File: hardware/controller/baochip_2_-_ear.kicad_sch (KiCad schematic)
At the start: 16 parts, among them U3 EA8212HT6R, U4 EA8212HT6R

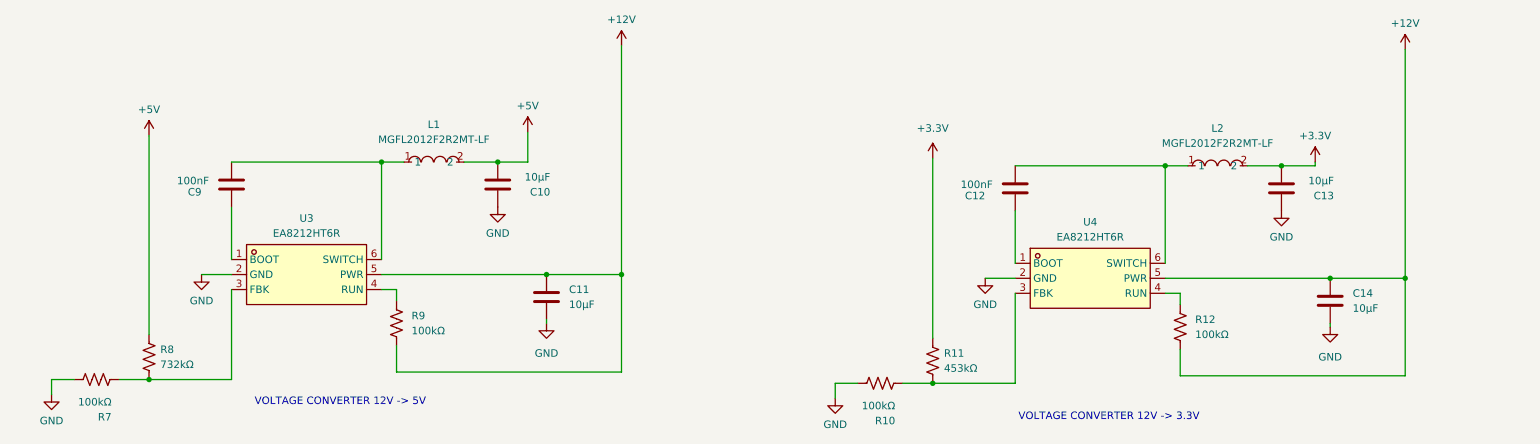
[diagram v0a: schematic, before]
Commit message: more controller board work, consolidation/revision of design
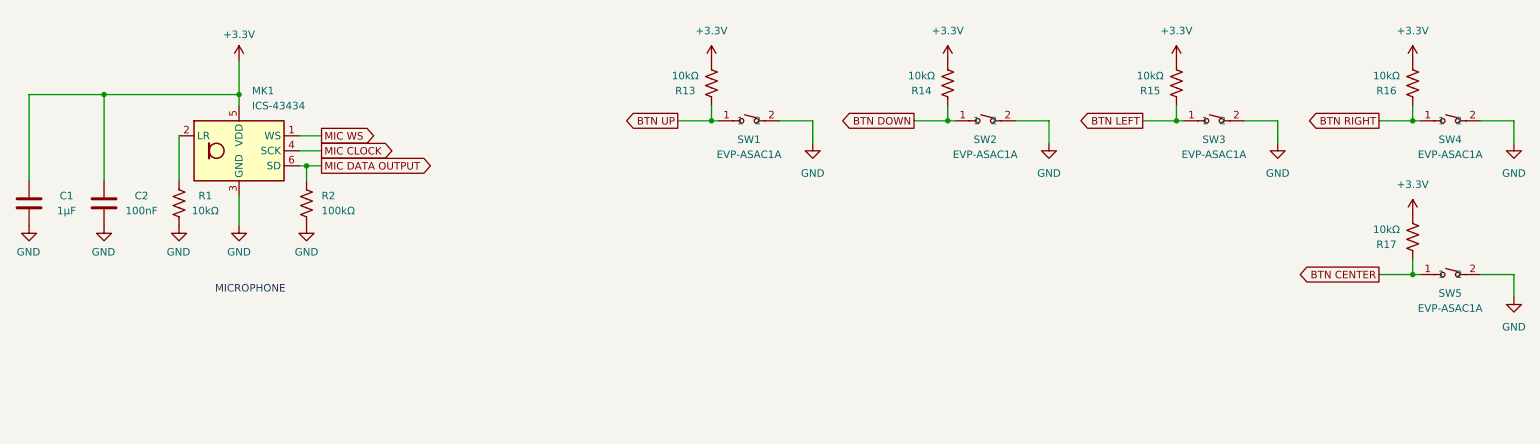
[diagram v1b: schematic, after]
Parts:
- removed C10, C11, C13, C14: 10µF, Capacitor_SMD:C_0603_1608Metric, symbol Device:C
- removed C12, C9: 100nF, Capacitor_SMD:C_0402_1005Metric, symbol Device:C
- removed L1, L2: MGFL2012F2R2MT-LF, footprints:L0805, symbol easyeda2kicad:MGFL2012F2R2MT-LF
- removed R10, R12, R7, R9: 100kΩ, Resistor_SMD:R_0402_1005Metric, symbol Device:R_US
- removed R11: 453kΩ, Resistor_SMD:R_0402_1005Metric, symbol Device:R_US
- removed R8: 732kΩ, Resistor_SMD:R_0402_1005Metric, symbol Device:R_US
- removed U3, U4: EA8212HT6R, footprints:SOT-23-6_L2.9-W1.6-P0.95-LS2.8-BR, symbol new:EA8212HT6R
- added C1: 1µF, Capacitor_SMD:C_0603_1608Metric, symbol Device:C
- added C2: 100nF, Capacitor_SMD:C_0402_1005Metric, symbol Device:C
- added MK1: ICS-43434, Sensor_Audio:InvenSense_ICS-43434-6_3.5x2.65mm, symbol Sensor_Audio:ICS-43434
- added R1, R13, R14, R15, R16, R17: 10kΩ, Resistor_SMD:R_0603_1608Metric, symbol Device:R_US
- added R2: 100kΩ, Resistor_SMD:R_0603_1608Metric, symbol Device:R_US
- added SW1, SW2, SW3, SW4, SW5: EVP-ASAC1A, easyeda2kicad:SW-SMD_PANASONIC_EVPASXXX, symbol easyeda2kicad:EVP-ASAC1A
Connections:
- net +3.3V: now also C1.1, C2.1, MK1.5 (VDD), R13.1, R14.1, R15.1, R16.1, R17.1
- net GND: now also C1.2, C2.2, MK1.3 (GND), R1.1, R2.1, SW1.2, SW2.2, SW3.2, SW4.2, SW5.2
- new net: MK1.2 (LR), R1.2
- new net BTN CENTER: R17.2, SW5.1
- new net BTN DOWN: R14.2, SW2.1
- new net BTN LEFT: R15.2, SW3.1
- new net BTN RIGHT: R16.2, SW4.1
- new net BTN UP: R13.2, SW1.1
- new net MIC CLOCK: MK1.4 (SCK)
- new net MIC DATA OUTPUT: MK1.6 (SD), R2.2
- new net MIC WS: MK1.1 (WS)
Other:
- note added: "MICROPHONE"
- note removed: "VOLTAGE CONVERTER 12V -> 3.3V"
- note removed: "VOLTAGE CONVERTER 12V -> 5V"
